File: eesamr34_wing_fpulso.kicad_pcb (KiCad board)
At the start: 2 copper layers, 50.9 x 25.6 mm, 12 parts, among them J3 Conn_01x02_Male, P1 SolderJumper_3_Bridged12, U2 4069

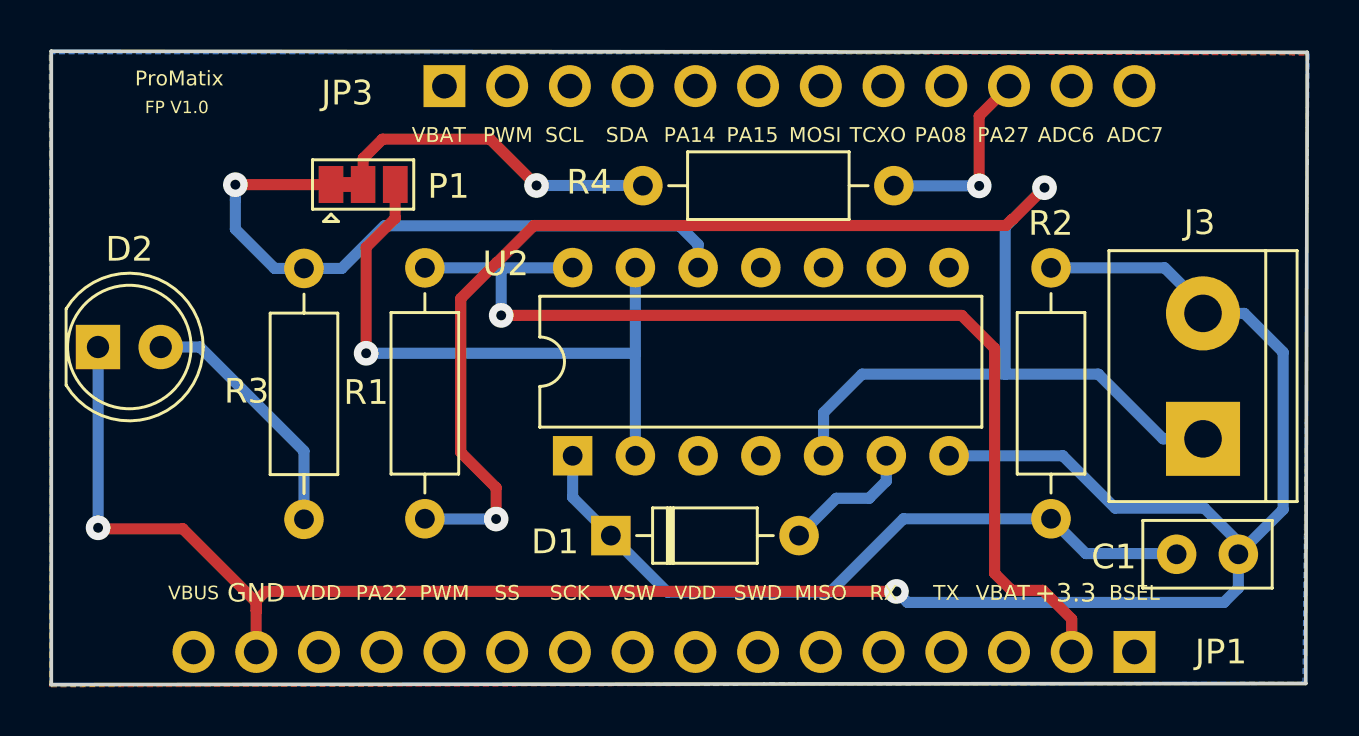
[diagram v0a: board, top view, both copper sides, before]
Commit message: Added ibom, gerbers
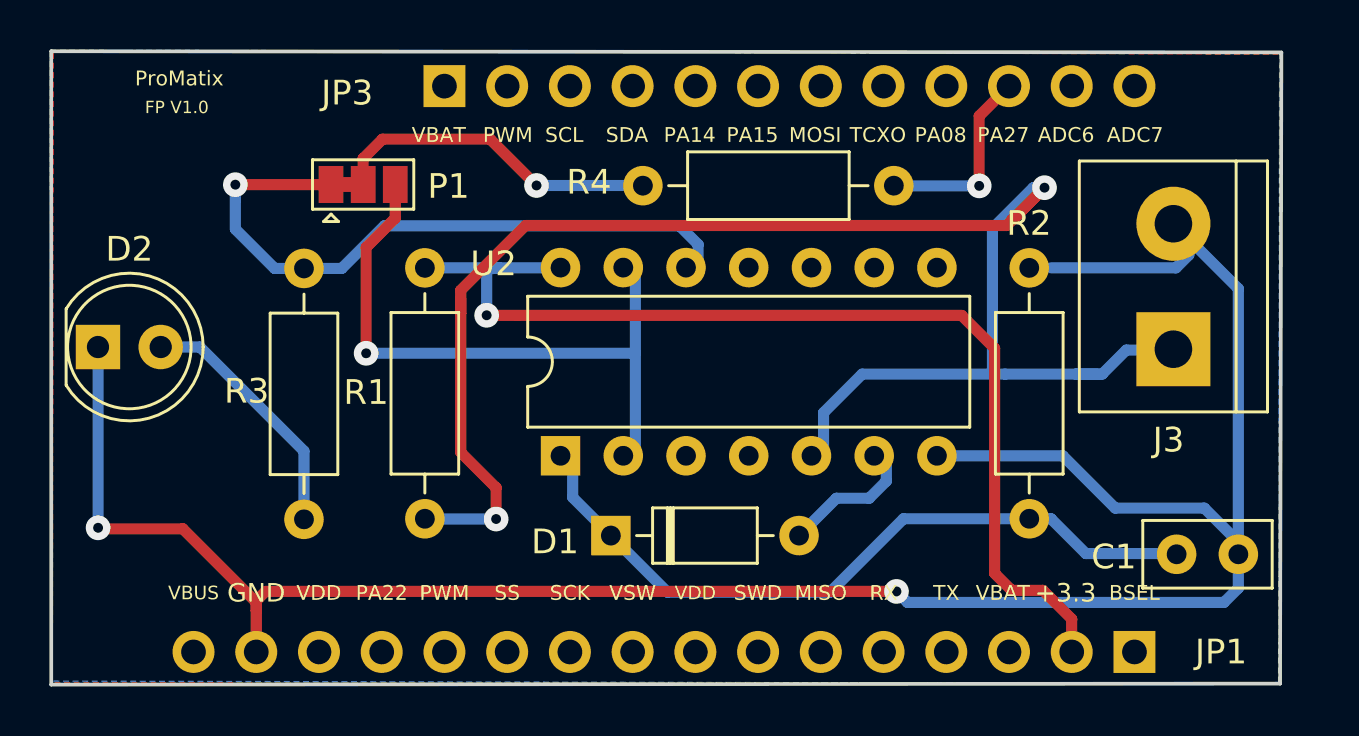
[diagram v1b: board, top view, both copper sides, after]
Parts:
- moved J3 3.82 mm to (70.9, 37.4)
- moved R2 0.88 mm to (65.1, 44.2)
- moved U2 0.49 mm to (46.1, 41.7)
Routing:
- net /Pulso: track 65.1 -> 67.9 mm
- net GND: track 93.0 -> 94.6 mm
- net /+3.3V: track 42.8 -> 43.8 mm
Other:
- board size 50.9 x 25.6 mm -> 49.8 x 25.6 mm
